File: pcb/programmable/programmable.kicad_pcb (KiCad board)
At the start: 2 copper layers, 88.6 x 167.9 mm, 91 parts, among them J1 AudioJack3_Ground, U1 Raspberry_Pi_Pico

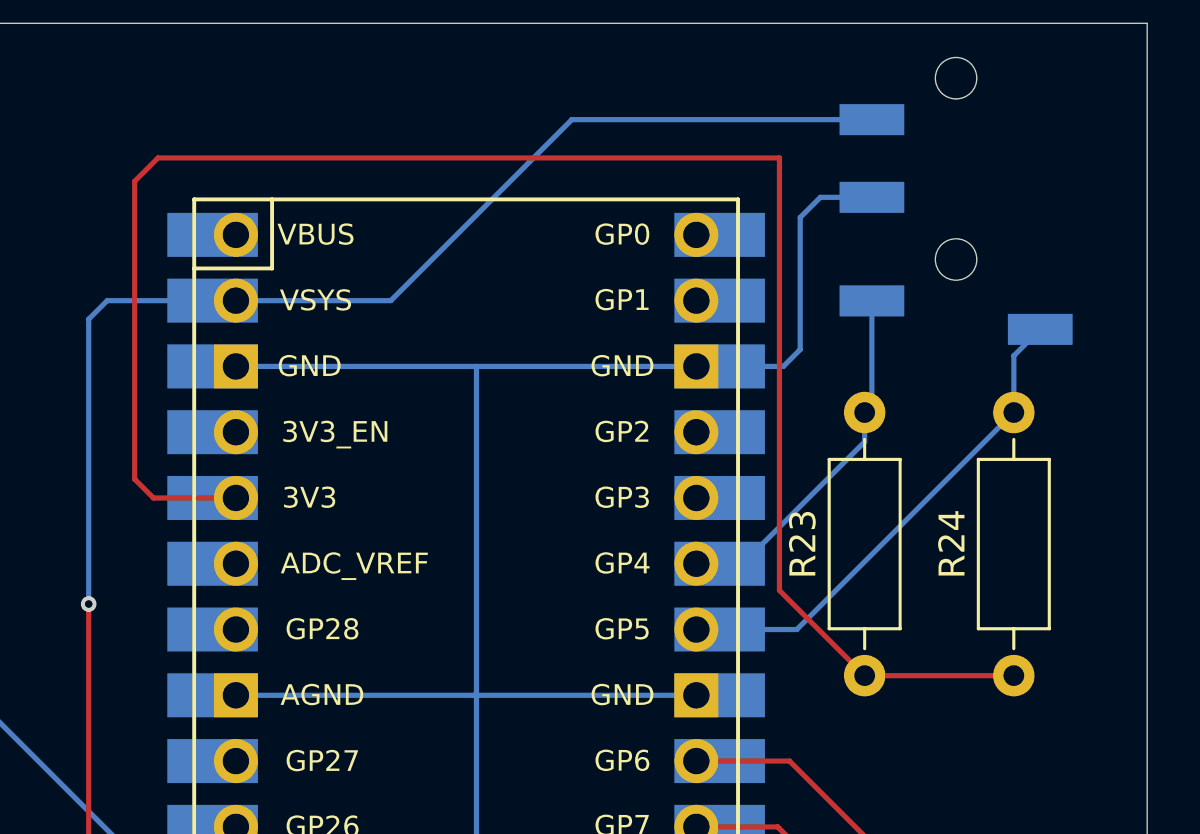
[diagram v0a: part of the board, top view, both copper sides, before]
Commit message: numerical done
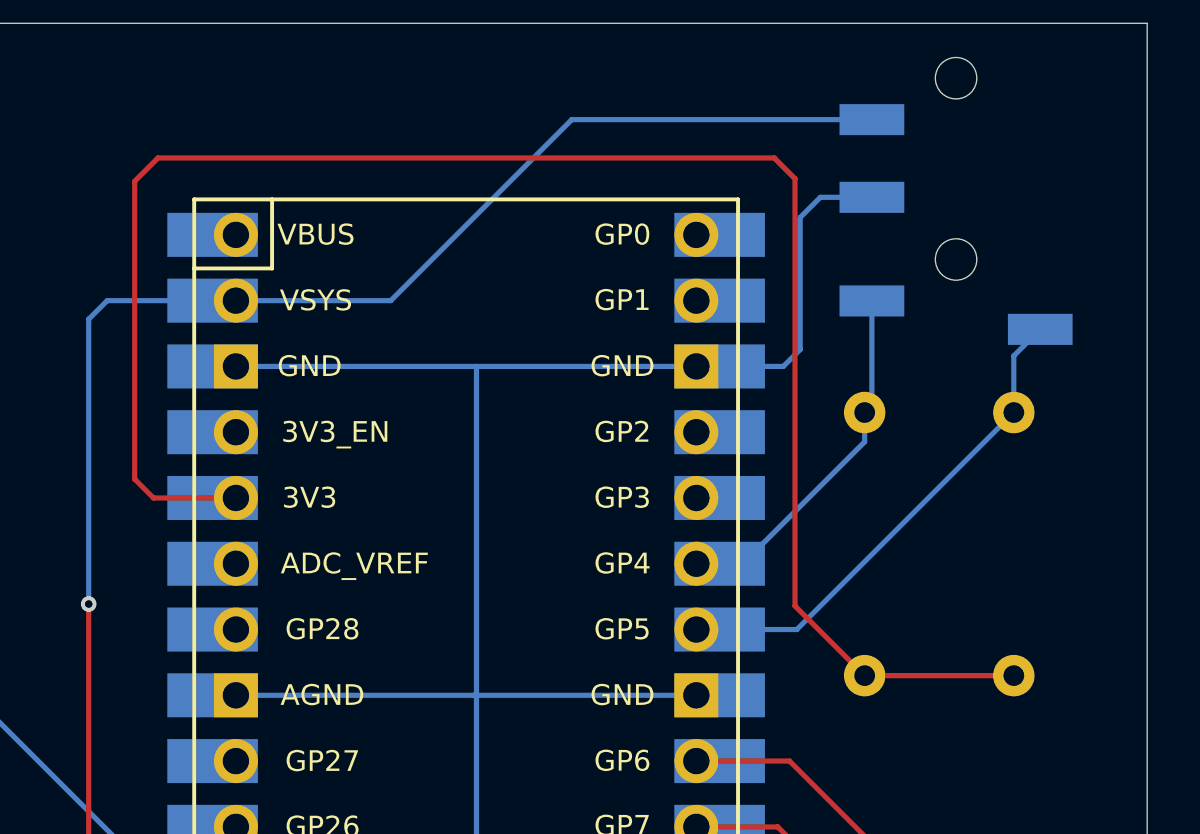
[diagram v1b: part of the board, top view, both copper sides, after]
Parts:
- R23, R24: moved to B.Cu
